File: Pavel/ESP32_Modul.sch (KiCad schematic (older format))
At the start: 1 part

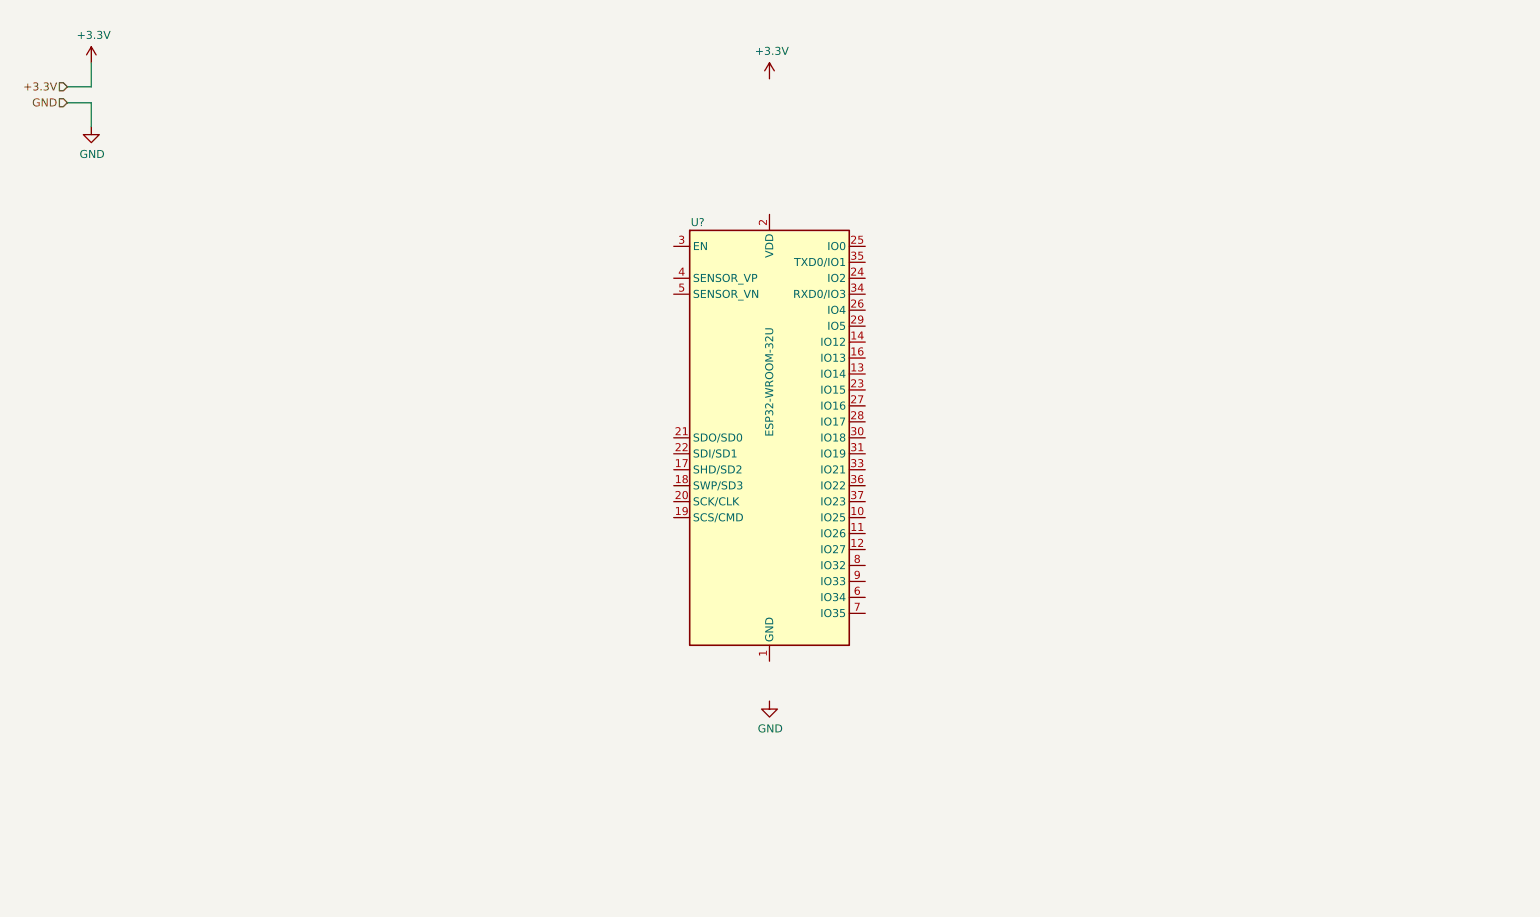
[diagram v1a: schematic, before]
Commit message: save commit again
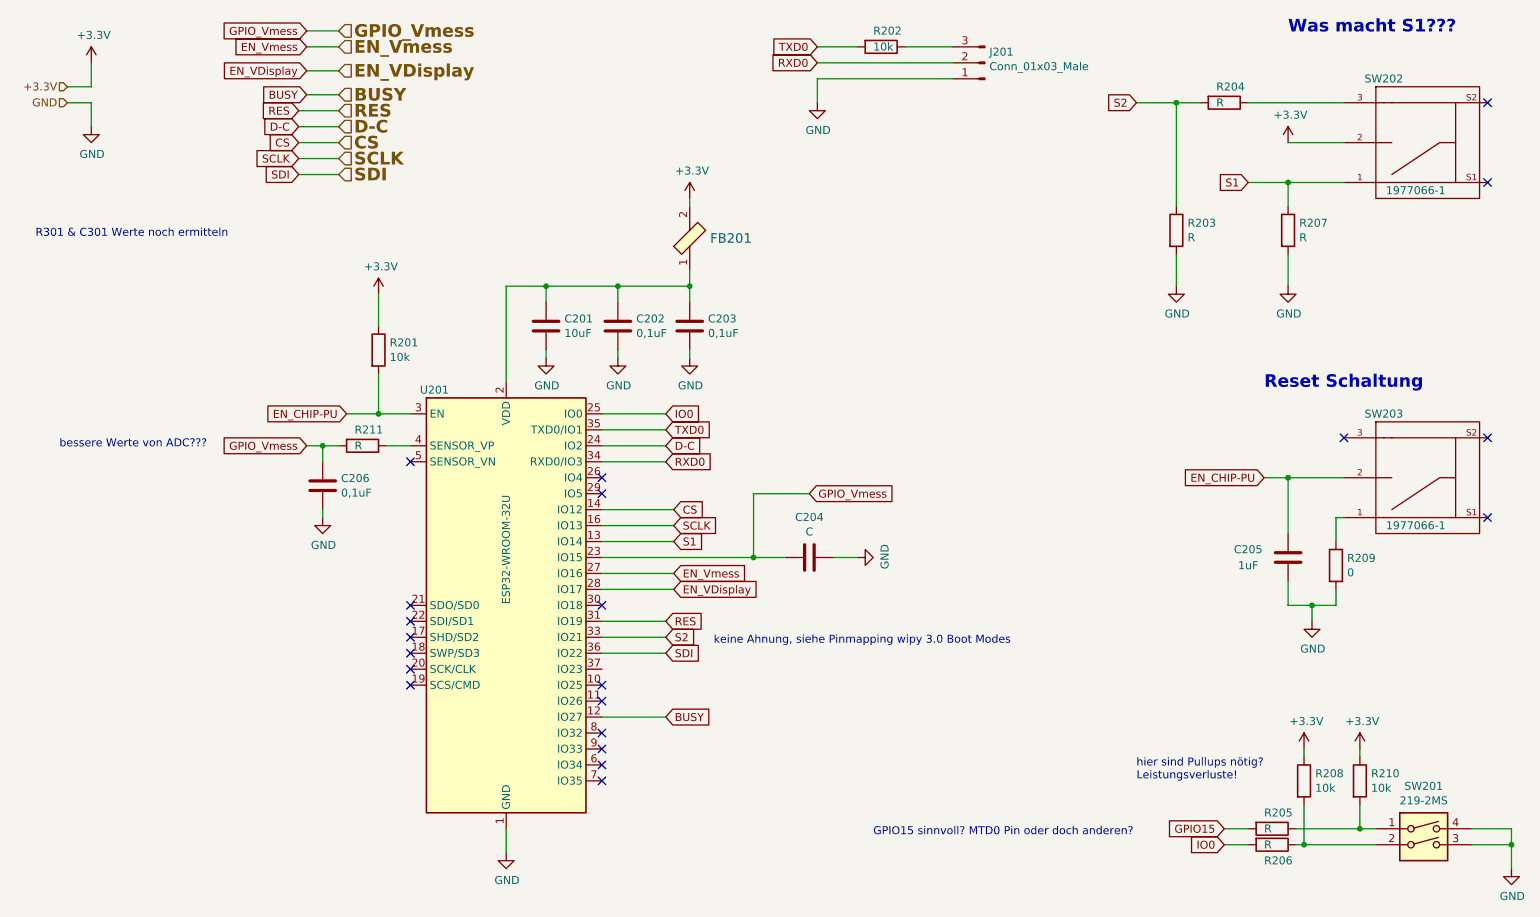
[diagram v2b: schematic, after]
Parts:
- added C201: 10uF, Capacitor_SMD:C_0603_1608Metric, symbol Device:C
- added C202, C203, C206: 0,1uF, Capacitor_SMD:C_0603_1608Metric, symbol Device:C
- added C204: C, Capacitor_SMD:C_0603_1608Metric, symbol Device:C
- added C205: 1uF, Capacitor_SMD:C_0603_1608Metric, symbol Device:C
- added FB201: 742792641, digikey-footprints:0603, symbol Pavel_privat:742792641
- added J201: Conn_01x03_Male, Connector:FanPinHeader_1x03_P2.54mm_Vertical, symbol Connector:Conn_01x03_Male
- added R201, R202, R208, R210: 10k, Resistor_SMD:R_0603_1608Metric_Pad1.05x0.95mm_HandSolder, symbol Device:R
- added R203, R204, R205, R206, R207, R211: R, Resistor_SMD:R_0603_1608Metric_Pad1.05x0.95mm_HandSolder, symbol Device:R
- added R209: 0, Resistor_SMD:R_0603_1608Metric_Pad1.05x0.95mm_HandSolder, symbol Device:R
- added SW201: 219-2MS, Button_Switch_SMD:SW_DIP_SPSTx02_Slide_6.7x6.64mm_W8.61mm_P2.54mm_LowProfile, symbol Pavel_privat:219-2MS
- added SW202, SW203: 1977066-1, Pavel_privat:TE_1977066-1, symbol Pavel_privat:1977066-1
- gave numbers to parts that had none: 1
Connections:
- net +3V3: now also FB201.2, R201.1, R208.1, R210.1, SW202.2
- net GND: now also U201.1 (GND), U201.15 (GND), U201.38 (GND), C201.2, C202.2, C203.2, C204.1, C205.1, C206.2, J201.1 (Pin_1), R203.2, R207.2, R209.2, SW201.3, SW201.4
- net BUSY: now reaches U201.12 (IO27)
- net S1: now reaches U201.13 (IO14)
- net S1: now also R207.1, SW202.1
- net CS: now reaches U201.14 (IO12)
- net SCLK: now reaches U201.16 (IO13)
- net at U201.2 (VDD): now also C201.1, C202.1, C203.1, FB201.1
- net GPIO_Vmess: now reaches U201.23 (IO15)
- net GPIO_Vmess: now also C204.2, C206.1, R211.2
- net D-C: now reaches U201.24 (IO2)
- net IO0: now reaches U201.25 (IO0)
- net IO0: now also R206.2
- net EN_Vmess: now reaches U201.27 (IO16)
- net EN_VDisplay: now reaches U201.28 (IO17)
- net EN_CHIP-PU: now reaches U201.3 (EN)
- net EN_CHIP-PU: now also C205.2, R201.2, SW203.2
- net RES: now reaches U201.31 (IO19)
- net S2: now reaches U201.33 (IO21)
- net S2: now also R203.1, R204.2
- net RXD0: now reaches U201.34 (RXD0/IO3)
- net RXD0: now also J201.2 (Pin_2)
- net TXD0: now reaches U201.35 (TXD0/IO1)
- net TXD0: now also R202.2
- net SDI: now reaches U201.36 (IO22)
- net at U201.4 (SENSOR_VP): now also R211.1
- new net: R205.1, R210.2, SW201.1
- new net: R206.1, R208.2, SW201.2
- new net: R204.1, SW202.3 (1)
- new net: R209.1, SW203.1
- new net: J201.3 (Pin_3), R202.1
- new net GPIO15: R205.2
- no-connect marks 0 -> 21
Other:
- note added: "GPIO15 sinnvoll? MTD0 Pin oder doch anderen?"
- note added: "R301 & C301 Werte noch ermitteln"
- note added: "Reset Schaltung\n"
- note added: "Was macht S1???\n\n"
- note added: "bessere Werte von ADC???\n\n"
- note added: "hier sind Pullups nötig?\nLeistungsverluste!"
- note added: "keine Ahnung, siehe Pinmapping wipy 3.0 Boot Modes\n"
- moved on the sheet: U201
